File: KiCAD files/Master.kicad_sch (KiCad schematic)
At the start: 24 parts, among them SW1 EG1271A, SW2 EG1271A, SW3 EG1271A, SW4 EG1271A, U4 NUCLEO64-F446RE

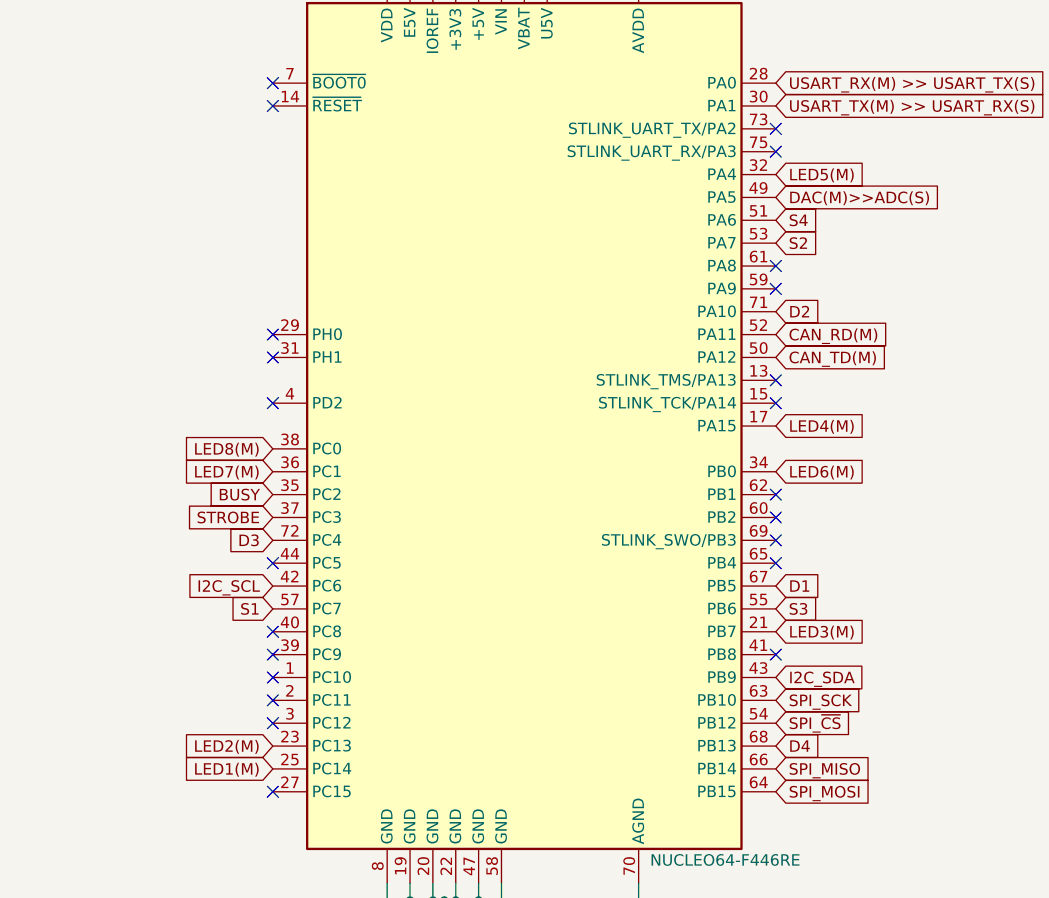
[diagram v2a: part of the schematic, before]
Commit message: update
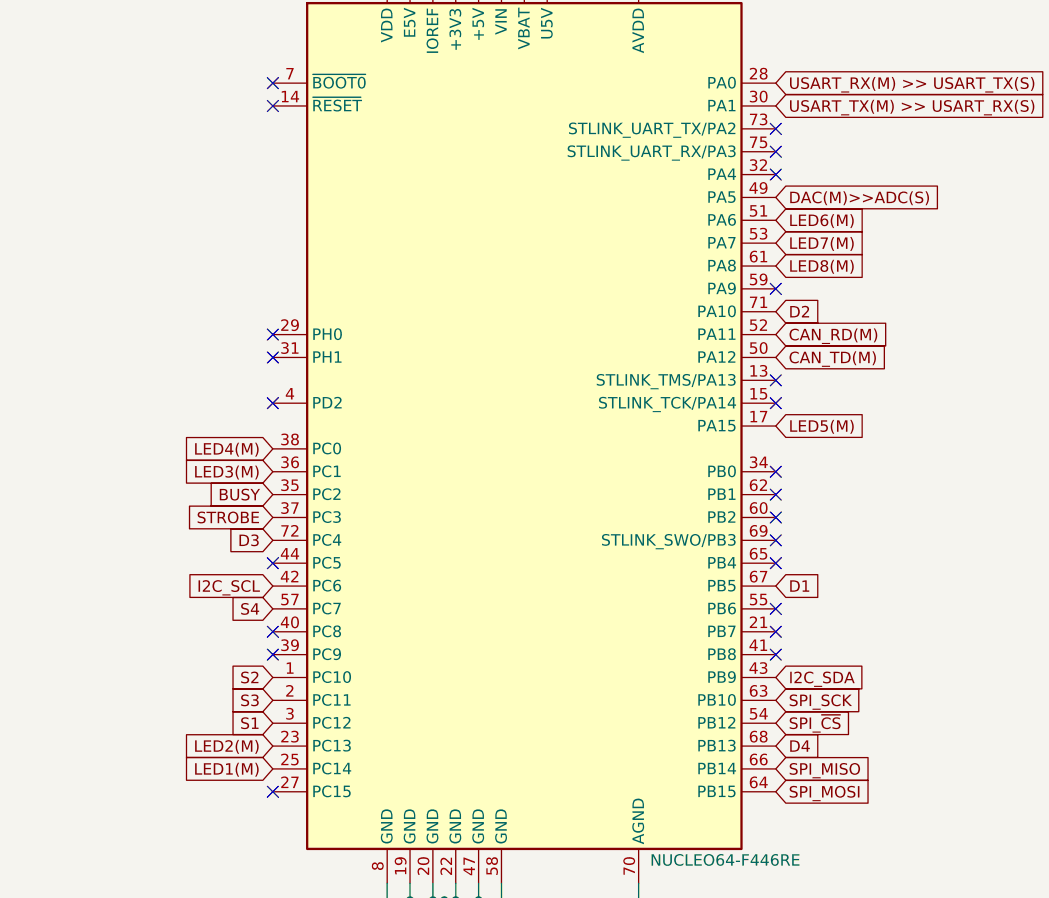
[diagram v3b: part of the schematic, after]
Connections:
- net LED3(M): now also U4.36 (PC1); no longer U4.21 (PB7)
- net LED4(M): now also U4.38 (PC0); no longer U4.17 (PA15)
- net LED5(M): now also U4.17 (PA15); no longer U4.32 (PA4)
- net LED6(M): now also U4.51 (PA6); no longer U4.34 (PB0)
- net LED7(M): now also U4.53 (PA7); no longer U4.36 (PC1)
- net LED8(M): now also U4.61 (PA8); no longer U4.38 (PC0)
- net S1: now also U4.3 (PC12); no longer U4.57 (PC7)
- net S2: now also U4.1 (PC10); no longer U4.53 (PA7)
- net S3: now also U4.2 (PC11); no longer U4.55 (PB6)
- net S4: now also U4.57 (PC7); no longer U4.51 (PA6)
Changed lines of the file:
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@@
   (junction (at 37.465 95.885) (diameter 0) (color 0 0 0 0)
   )
-  (no_connect (at 169.545 73.66))
+  (no_connect (at 169.545 111.76))
   (no_connect (at 169.545 106.68))
   (no_connect (at 57.785 136.525))
@@
   (no_connect (at 169.545 104.14))
   (no_connect (at 139.065 40.64))
+  (no_connect (at 169.545 114.3))
   (no_connect (at 58.42 125.73))
   (no_connect (at 169.545 60.96))
   (no_connect (at 154.305 40.64))
-  (no_connect (at 113.665 124.46))
   (no_connect (at 144.145 40.64))
   (no_connect (at 131.445 40.64))
@@
   (no_connect (at 133.985 40.64))
   (no_connect (at 169.545 58.42))
-  (no_connect (at 113.665 119.38))
-  (no_connect (at 113.665 121.92))
+  (no_connect (at 169.545 63.5))
   (no_connect (at 128.905 40.64))
   (no_connect (at 113.665 88.9))
   (no_connect (at 169.545 99.06))
+  (no_connect (at 169.545 96.52))
   (no_connect (at 113.665 132.08))
   (no_connect (at 169.545 76.2))
@@
     (effects (font (size 1.27 1.27)) (justify left bottom))
   )
-  (global_label "S3" (shape input) (at 169.545 111.76 0) (fields_autoplaced)
-    (effects (font (size 1.27 1.27)) (justify left))
-    (property "Intersheetrefs" "${INTERSHEET_REFS}" (at 174.9492 111.76 0)
-      (effects (font (size 1.27 1.27)) (justify left) hide)
+  (global_label "S3" (shape input) (at 113.665 121.92 180) (fields_autoplaced)
+    (effects (font (size 1.27 1.27)) (justify right))
+    (property "Intersheetrefs" "${INTERSHEET_REFS}" (at 108.2608 121.92 0)
+      (effects (font (size 1.27 1.27)) (justify right) hide)
     )
   )
@@
     )
   )
-  (global_label "LED5(M)" (shape input) (at 169.545 63.5 0) (fields_autoplaced)
-    (effects (font (size 1.27 1.27)) (justify left))
-    (property "Intersheetrefs" "${INTERSHEET_REFS}" (at 180.3316 63.5 0)
+  (global_label "LED5(M)" (shape input) (at 169.545 91.44 0) (fields_autoplaced)
+    (effects (font (size 1.27 1.27)) (justify left))
+    (property "Intersheetrefs" "${INTERSHEET_REFS}" (at 180.3316 91.44 0)
       (effects (font (size 1.27 1.27)) (justify left) hide)
     )
@@
     )
   )
-  (global_label "S2" (shape input) (at 169.545 71.12 0) (fields_autoplaced)
-    (effects (font (size 1.27 1.27)) (justify left))
-    (property "Intersheetrefs" "${INTERSHEET_REFS}" (at 174.9492 71.12 0)
-      (effects (font (size 1.27 1.27)) (justify left) hide)
-    )
-  )
-  (global_label "S4" (shape input) (at 169.545 68.58 0) (fields_autoplaced)
-    (effects (font (size 1.27 1.27)) (justify left))
-    (property "Intersheetrefs" "${INTERSHEET_REFS}" (at 174.9492 68.58 0)
-      (effects (font (size 1.27 1.27)) (justify left) hide)
+  (global_label "S2" (shape input) (at 113.665 119.38 180) (fields_autoplaced)
+    (effects (font (size 1.27 1.27)) (justify right))
+    (property "Intersheetrefs" "${INTERSHEET_REFS}" (at 108.2608 119.38 0)
+      (effects (font (size 1.27 1.27)) (justify right) hide)
+    )
+  )
+  (global_label "S4" (shape input) (at 113.665 111.76 180) (fields_autoplaced)
+    (effects (font (size 1.27 1.27)) (justify right))
+    (property "Intersheetrefs" "${INTERSHEET_REFS}" (at 108.2608 111.76 0)
+      (effects (font (size 1.27 1.27)) (justify right) hide)
     )
   )
@@
     )
   )
-  (global_label "LED3(M)" (shape input) (at 169.545 114.3 0) (fields_autoplaced)
-    (effects (font (size 1.27 1.27)) (justify left))
-    (property "Intersheetrefs" "${INTERSHEET_REFS}" (at 180.3316 114.3 0)
-      (effects (font (size 1.27 1.27)) (justify left) hide)
+  (global_label "LED3(M)" (shape input) (at 113.665 96.52 180) (fields_autoplaced)
+    (effects (font (size 1.27 1.27)) (justify right))
+    (property "Intersheetrefs" "${INTERSHEET_REFS}" (at 102.8784 96.52 0)
+      (effects (font (size 1.27 1.27)) (justify right) hide)
     )
   )
@@
     )
   )
-  (global_label "LED8(M)" (shape input) (at 113.665 93.98 180) (fields_autoplaced)
+  (global_label "LED8(M)" (shape input) (at 169.545 73.66 0) (fields_autoplaced)
+    (effects (font (size 1.27 1.27)) (justify left))
+    (property "Intersheetrefs" "${INTERSHEET_REFS}" (at 180.3316 73.66 0)
+      (effects (font (size 1.27 1.27)) (justify left) hide)
+    )
+  )
+  (global_label "LED6(M)" (shape input) (at 169.545 68.58 0) (fields_autoplaced)
+    (effects (font (size 1.27 1.27)) (justify left))
+    (property "Intersheetrefs" "${INTERSHEET_REFS}" (at 180.3316 68.58 0)
+      (effects (font (size 1.27 1.27)) (justify left) hide)
+    )
+  )
+  (global_label "DAC(M)>>ADC(S)" (shape input) (at 107.95 172.085 0) (fields_autoplaced)
+    (effects (font (size 1.27 1.27)) (justify left))
+    (property "Intersheetrefs" "${INTERSHEET_REFS}" (at 127.3849 172.085 0)
+      (effects (font (size 1.27 1.27)) (justify left) hide)
+    )
+  )
+  (global_label "S1" (shape input) (at 48.26 128.27 180) (fields_autoplaced)
+    (effects (font (size 1.27 1.27)) (justify right))
+    (property "Intersheetrefs" "${INTERSHEET_REFS}" (at 42.8558 128.27 0)
+      (effects (font (size 1.27 1.27)) (justify right) hide)
+    )
+  )
+  (global_label "LED5(M)" (shape input) (at 20.955 82.55 90) (fields_autoplaced)
+    (effects (font (size 1.27 1.27)) (justify left))
+    (property "Intersheetrefs" "${INTERSHEET_REFS}" (at 20.955 71.7634 90)
+      (effects (font (size 1.27 1.27)) (justify left) hide)
+    )
+  )
+  (global_label "BUSY" (shape input) (at 113.665 99.06 180) (fields_autoplaced)
+    (effects (font (size 1.27 1.27)) (justify right))
+    (property "Intersheetrefs" "${INTERSHEET_REFS}" (at 105.7812 99.06 0)
+      (effects (font (size 1.27 1.27)) (justify right) hide)
+    )
+  )
+  (global_label "LED1(M)" (shape input) (at 20.32 38.1 90) (fields_autoplaced)
+    (effects (font (size 1.27 1.27)) (justify left))
+    (property "Intersheetrefs" "${INTERSHEET_REFS}" (at 20.32 27.3134 90)
+      (effects (font (size 1.27 1.27)) (justify left) hide)
+    )
+  )
+  (global_label "LED4(M)" (shape input) (at 113.665 93.98 180) (fields_autoplaced)
     (effects (font (size 1.27 1.27)) (justify right))
     (property "Intersheetrefs" "${INTERSHEET_REFS}" (at 102.8784 93.98 0)
@@
     )
   )
-  (global_label "LED6(M)" (shape input) (at 169.545 96.52 0) (fields_autoplaced)
-    (effects (font (size 1.27 1.27)) (justify left))
-    (property "Intersheetrefs" "${INTERSHEET_REFS}" (at 180.3316 96.52 0)
-      (effects (font (size 1.27 1.27)) (justify left) hide)
-    )
-  )
-  (global_label "DAC(M)>>ADC(S)" (shape input) (at 107.95 172.085 0) (fields_autoplaced)
-    (effects (font (size 1.27 1.27)) (justify left))
-    (property "Intersheetrefs" "${INTERSHEET_REFS}" (at 127.3849 172.085 0)
-      (effects (font (size 1.27 1.27)) (justify left) hide)
-    )
-  )
-  (global_label "S1" (shape input) (at 48.26 128.27 180) (fields_autoplaced)
-    (effects (font (size 1.27 1.27)) (justify right))
-    (property "Intersheetrefs" "${INTERSHEET_REFS}" (at 42.8558 128.27 0)
-      (effects (font (size 1.27 1.27)) (justify right) hide)
-    )
-  )
-  (global_label "LED5(M)" (shape input) (at 20.955 82.55 90) (fields_autoplaced)
-    (effects (font (size 1.27 1.27)) (justify left))
-    (property "Intersheetrefs" "${INTERSHEET_REFS}" (at 20.955 71.7634 90)
-      (effects (font (size 1.27 1.27)) (justify left) hide)
-    )
-  )
-  (global_label "BUSY" (shape input) (at 113.665 99.06 180) (fields_autoplaced)
-    (effects (font (size 1.27 1.27)) (justify right))
-    (property "Intersheetrefs" "${INTERSHEET_REFS}" (at 105.7812 99.06 0)
-      (effects (font (size 1.27 1.27)) (justify right) hide)
-    )
-  )
-  (global_label "LED1(M)" (shape input) (at 20.32 38.1 90) (fields_autoplaced)
-    (effects (font (size 1.27 1.27)) (justify left))
-    (property "Intersheetrefs" "${INTERSHEET_REFS}" (at 20.32 27.3134 90)
-      (effects (font (size 1.27 1.27)) (justify left) hide)
-    )
-  )
-  (global_label "LED4(M)" (shape input) (at 169.545 91.44 0) (fields_autoplaced)
-    (effects (font (size 1.27 1.27)) (justify left))
-    (property "Intersheetrefs" "${INTERSHEET_REFS}" (at 180.3316 91.44 0)
-      (effects (font (size 1.27 1.27)) (justify left) hide)
-    )
-  )
   (global_label "S2" (shape input) (at 47.625 139.065 180) (fields_autoplaced)
     (effects (font (size 1.27 1.27)) (justify right))
@@
     )
   )
-  (global_label "LED7(M)" (shape input) (at 113.665 96.52 180) (fields_autoplaced)
-    (effects (font (size 1.27 1.27)) (justify right))
-    (property "Intersheetrefs" "${INTERSHEET_REFS}" (at 102.8784 96.52 0)
-      (effects (font (size 1.27 1.27)) (justify right) hide)
+  (global_label "LED7(M)" (shape input) (at 169.545 71.12 0) (fields_autoplaced)
+    (effects (font (size 1.27 1.27)) (justify left))
+    (property "Intersheetrefs" "${INTERSHEET_REFS}" (at 180.3316 71.12 0)
+      (effects (font (size 1.27 1.27)) (justify left) hide)
     )
   )
@@
     )
   )
-  (global_label "S1" (shape input) (at 113.665 111.76 180) (fields_autoplaced)
-    (effects (font (size 1.27 1.27)) (justify right))
-    (property "Intersheetrefs" "${INTERSHEET_REFS}" (at 108.2608 111.76 0)
-      (effects (font (size 1.27 1.27)) (justify right) hide)
-    )
+  (global_label "S1" (shape input) (at 113.665 124.46 180) (fields_autoplaced)
+    (effects (font (size 1.27 1.27)) (justify right))
+    (property "Intersheetrefs" "${INTERSHEET_REFS}" (at 108.2608 124.46 0)
+      (effects (font (size 1.27 1.27)) (justify right) hide)
+    )
